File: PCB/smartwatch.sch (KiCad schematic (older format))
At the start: 55 parts, among them U1 STM32F103C8T6, U2 HM-10_MIN, U3 M25P40, U4 BMC150, U5 BMP180, U6 STC4054, U7 NCP551, U8 UG-2864HSWEG01, X1 PLS1, X2 PLS1, X3 PLS1, X4 PLS1, X5 PLS1, X6 PLS1

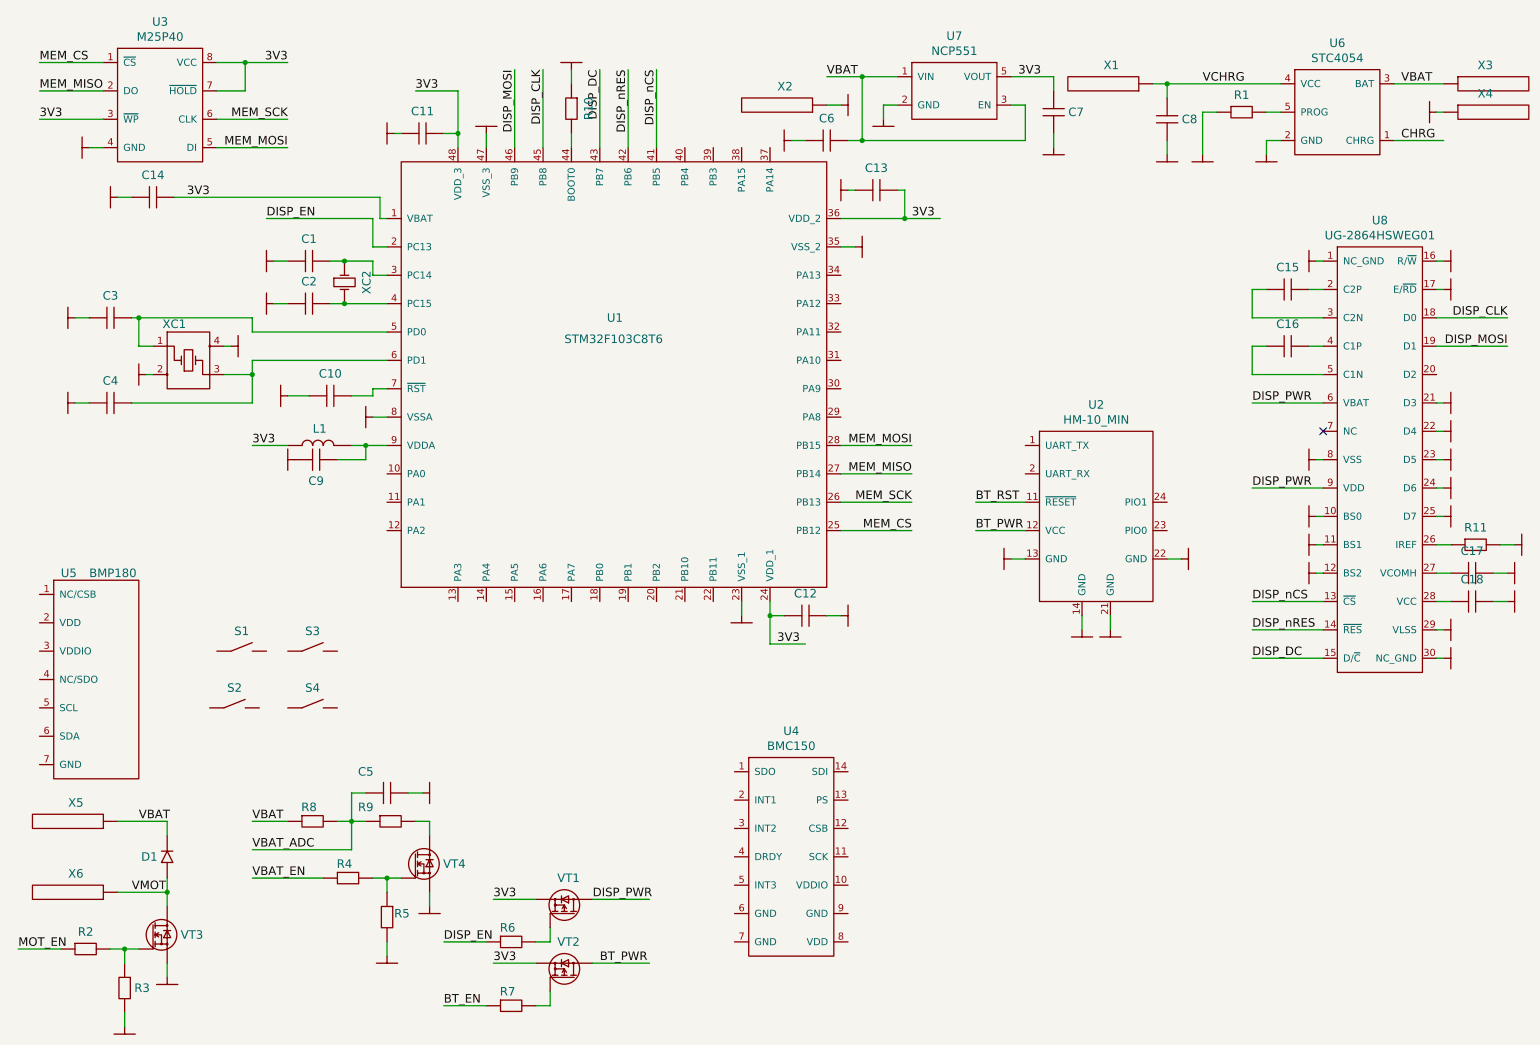
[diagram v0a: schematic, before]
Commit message: PCB (everything is done, should be checked)
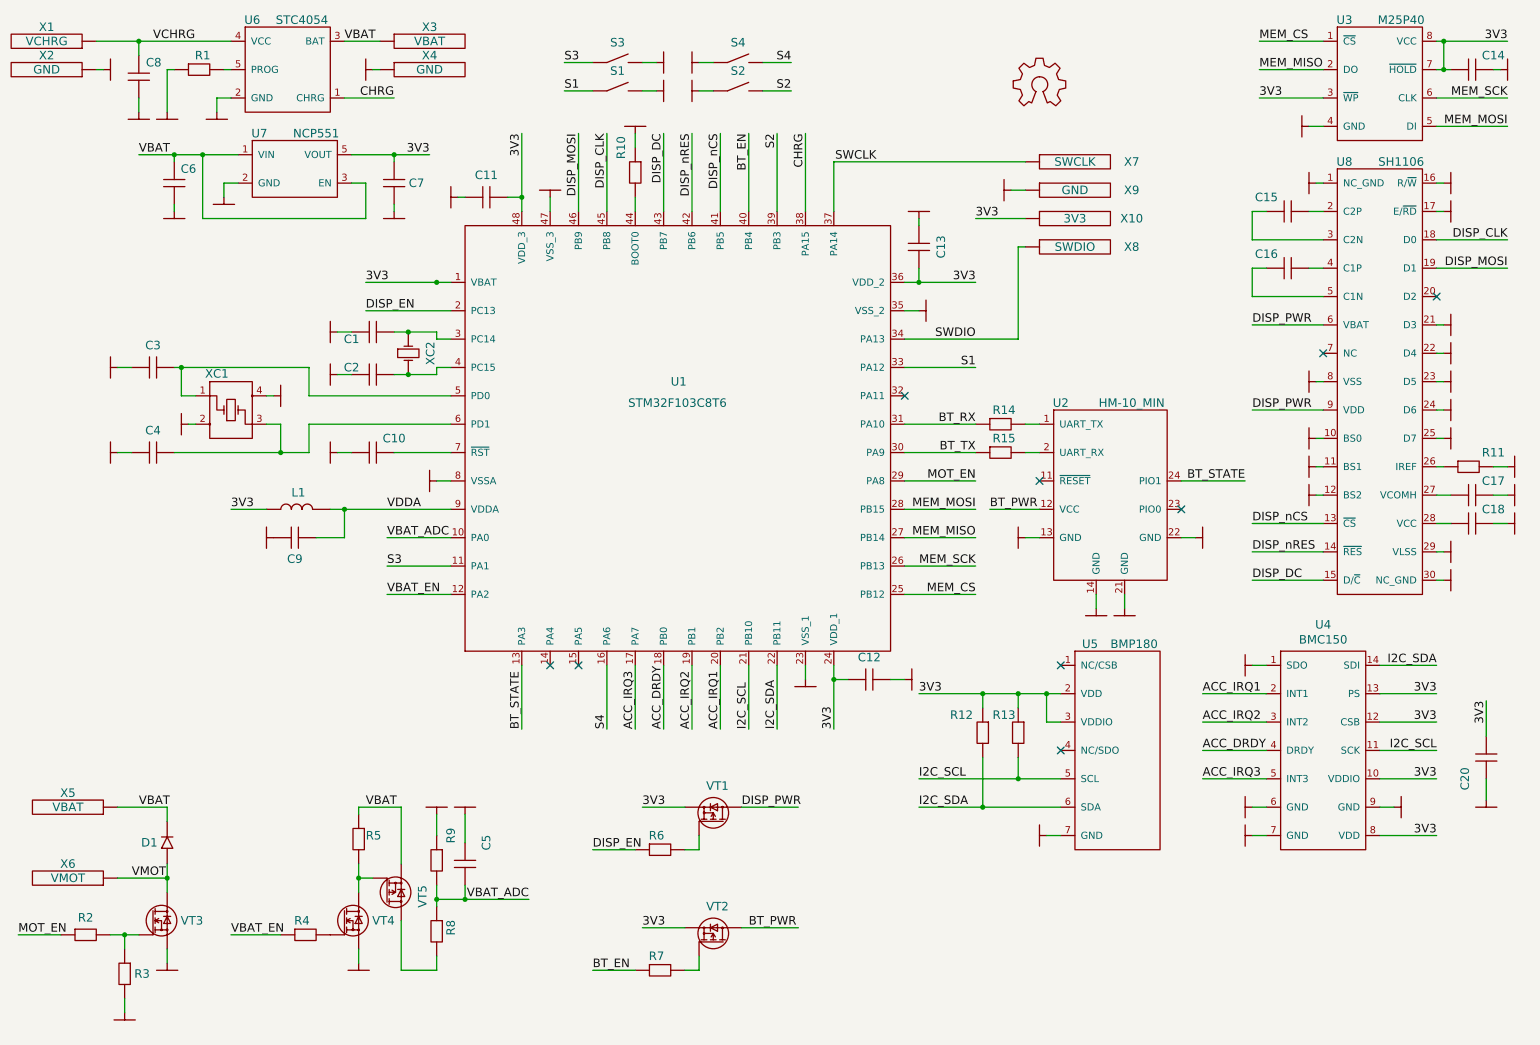
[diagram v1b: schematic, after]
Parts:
- added C20: capacitor, discrete_SMD:0402_C, symbol capacitor
- added LG?1: LOGO, LOGO:OSHW, symbol LOGO
- added R12, R13: resistor, discrete_SMD:0402_R, symbol resistor
- added R14, R15: 390k, discrete_SMD:0402_R, symbol resistor
- added VT5: MOSFET_P_DGS, IR:PQFN2x2, symbol MOSFET_P_DGS
- added X10: 3V3, CONNECTORS:SLD_POINT, symbol PLS1
- added X7: SWCLK, CONNECTORS:SLD_POINT, symbol PLS1
- added X8: SWDIO, CONNECTORS:SLD_POINT, symbol PLS1
- added X9: GND, CONNECTORS:SLD_POINT, symbol PLS1
- U8: value UG-2864HSWEG01 -> SH1106
- X1: value PLS1 -> VCHRG
- X2, X4: value PLS1 -> GND
- X3, X5: value PLS1 -> VBAT
- X6: value PLS1 -> VMOT
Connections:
- net 3V3: now also U4.10 (VDDIO), U4.12 (CSB), U4.13 (PS), U4.8 (VDD), U5.2 (VDD), U5.3 (VDDIO), C20.2, R12.1, R13.1, X10.1
- net BT_EN: now also U1.40 (PB4)
- net CHRG: now also U1.38 (PA15)
- net GND: now also C5.1, R9.1, S1.2, S2.1, S3.2, S4.1, U4.1 (SDO), U4.6 (GND), U4.7 (GND), U4.9 (GND), U5.7 (GND), C20.1, X9.1; no longer C5.2, R5.2
- net MOT_EN: now also U1.29 (PA8)
- net VBAT: now also R5.1, VT5.3 (S); no longer R8.1
- net VBAT_ADC: now also C5.2, R8.1, R9.2, U1.10 (PA0); no longer C5.1, R8.2, R9.1
- net VBAT_EN: now also U1.12 (PA2)
- net VDDA: now reaches C9.2, L1.2, U1.9 (VDDA)
- net S3: now reaches U1.11 (PA1)
- net S3: now also S3.1
- net BT_STATE: now reaches U1.13 (PA3)
- net BT_STATE: now also U2.24 (PIO1)
- net S4: now reaches U1.16 (PA6)
- net S4: now also S4.2
- net ACC_IRQ3: now reaches U1.17 (PA7)
- net ACC_IRQ3: now also U4.5 (INT3)
- net ACC_DRDY: now reaches U1.18 (PB0)
- net ACC_DRDY: now also U4.4 (DRDY)
- net ACC_IRQ2: now reaches U1.19 (PB1)
- net ACC_IRQ2: now also U4.3 (INT2)
- net ACC_IRQ1: now reaches U1.20 (PB2)
- net ACC_IRQ1: now also U4.2 (INT1)
- net I2C_SCL: now reaches U1.21 (PB10)
- net I2C_SCL: now also U4.11 (SCK), U5.5 (SCL), R13.2
- net I2C_SDA: now reaches U1.22 (PB11)
- net I2C_SDA: now also U4.14 (SDI), U5.6 (SDA), R12.2
- net BT_TX: now reaches U1.30 (PA9)
- net BT_TX: now also R15.1
- net BT_RX: now reaches U1.31 (PA10)
- net BT_RX: now also R14.1
- net S1: now reaches U1.33 (PA12)
- net S1: now also S1.1
- net SWDIO: now reaches U1.34 (PA13)
- net SWDIO: now also X8.1
- net SWCLK: now reaches U1.37 (PA14)
- net SWCLK: now also X7.1
- net S2: now reaches U1.39 (PB3)
- net S2: now also S2.2
- net at VT4.1 (D): now also R5.2, VT5.2 (G); no longer R9.2
- net at R4.2, VT4.2 (G): no longer R5.1
- net at U2.1 (UART_TX): now also R14.2
- net at U2.2 (UART_RX): now also R15.2
- net BT_RST: no longer names the net of U2.11 (~RESET)
- new net: R8.2, VT5.1 (D)
- no-connect marks 1 -> 9
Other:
- moved on the sheet: C1, C10, C11, C12, C13, C14, C15, C16, C17, C18, C2, C3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
